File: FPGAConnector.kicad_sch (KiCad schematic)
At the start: 5 parts, among them J4 Conn_02x06_Counter_Clockwise, J5 Conn_02x07_Vertical, J6 To The Zedboard, J8 Conn_02x06_Odd_Even, J9 Conn_02x05_Counter_Clockwise

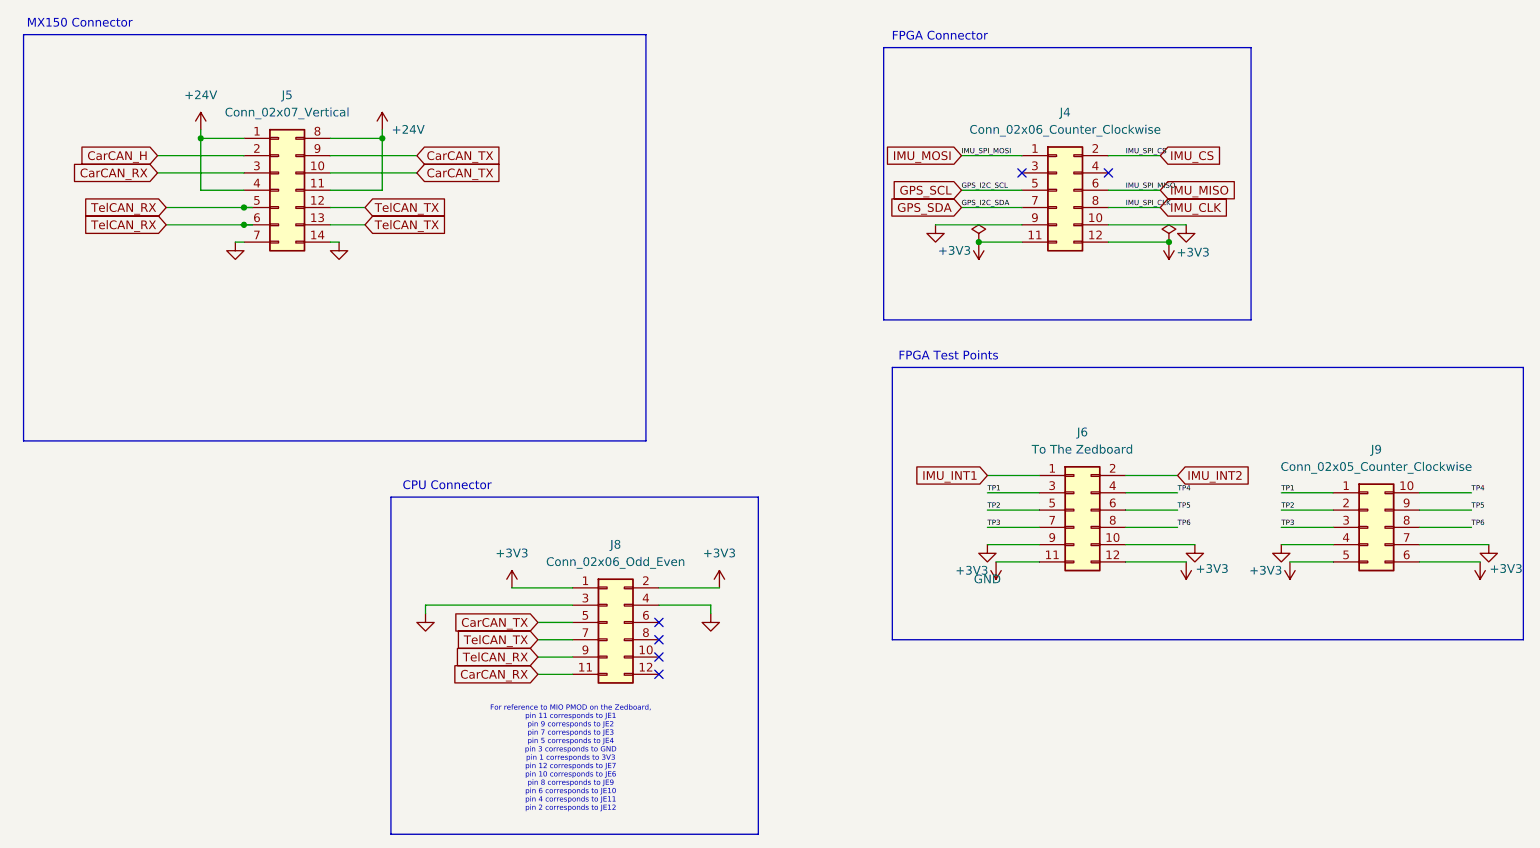
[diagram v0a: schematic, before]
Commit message: more layout
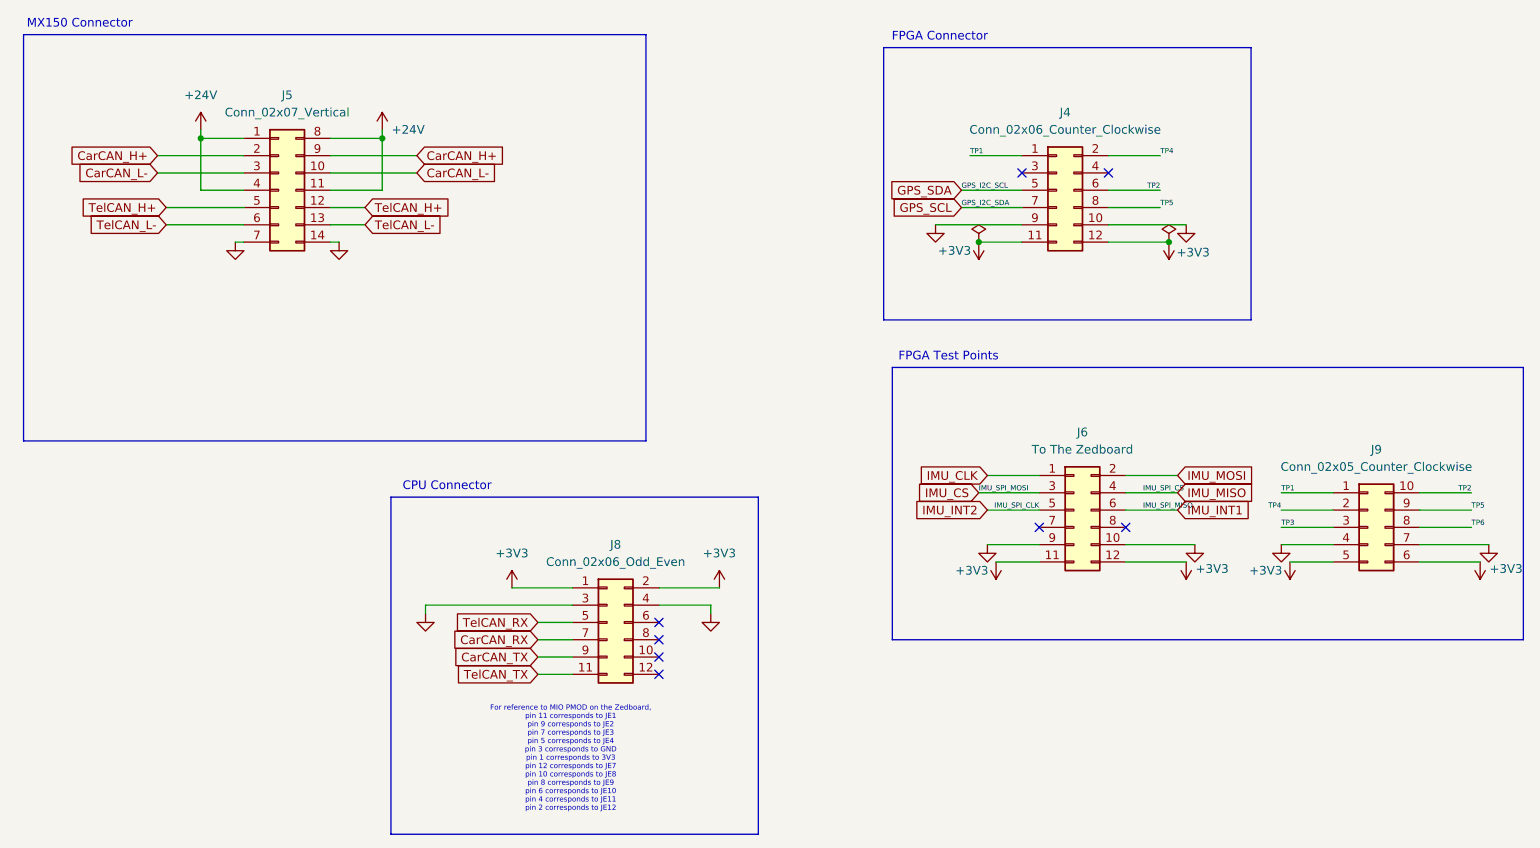
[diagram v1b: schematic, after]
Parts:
- J4: footprint Connector_PinHeader_2.54mm:PinHeader_2x07_P2.54mm_Vertical -> Connector_PinHeader_2.54mm:PinHeader_2x06_P2.54mm_Vertical
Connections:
- net CarCAN_RX: now also J8.7 (Pin_7); no longer J5.3 (Pin_3), J8.11 (Pin_11)
- net CarCAN_TX: now also J8.9 (Pin_9); no longer J5.10 (Pin_10), J5.9 (Pin_9), J8.5 (Pin_5)
- net GPS_SCL: now also J4.7 (Pin_7); no longer J4.5 (Pin_5)
- net GPS_SDA: now also J4.5 (Pin_5); no longer J4.7 (Pin_7)
- net IMU_CLK: now also J6.1 (Pin_1); no longer J4.8 (Pin_8)
- net IMU_CS: now also J6.3 (Pin_2); no longer J4.2 (Pin_2)
- net IMU_INT1: now also J6.6 (Pin_6); no longer J6.1 (Pin_1)
- net IMU_INT2: now also J6.5 (Pin_5); no longer J6.2 (Pin_2)
- net IMU_MISO: now also J6.4 (Pin_4); no longer J4.6 (Pin_6)
- net IMU_MOSI: now also J6.2 (Pin_2); no longer J4.1 (Pin_1)
- net TP1: now also J4.1 (Pin_1); no longer J6.3 (Pin_2)
- net TP2: now also J4.6 (Pin_6), J9.10 (Pin_10); no longer J6.5 (Pin_5), J9.2 (Pin_2)
- net TP3: no longer J6.7 (Pin_7)
- net TP4: now also J4.2 (Pin_2), J9.2 (Pin_2); no longer J6.4 (Pin_4), J9.10 (Pin_10)
- net TP5: now also J4.8 (Pin_8); no longer J6.6 (Pin_6)
- net TP6: no longer J6.8 (Pin_8)
- net TelCAN_RX: now also J8.5 (Pin_5); no longer J5.5 (Pin_5), J5.6 (Pin_6), J8.9 (Pin_9)
- net TelCAN_TX: now also J8.11 (Pin_11); no longer J5.12 (Pin_12), J5.13 (Pin_13), J8.7 (Pin_7)
- net CarCAN_H renamed CarCAN_H+
- net CarCAN_H+: now also J5.9 (Pin_9)
- new net CarCAN_L-: J5.10 (Pin_10), J5.3 (Pin_3)
- new net TelCAN_H+: J5.12 (Pin_12), J5.5 (Pin_5)
- new net TelCAN_L-: J5.13 (Pin_13), J5.6 (Pin_6)
- no-connect marks 6 -> 8
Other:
- note added: "For reference to MIO PMOD on the Zedboard, pin 11 corresponds to JE1 pin 9 corresponds to JE2 pin 7 corresponds to JE3 pin 5 corresponds to JE4 pin 3 corresponds to GND pin 1 corresponds to 3V3 pin 12 corresponds to JE7 pin 10 corresponds to JE8 pin 8 corresponds to JE9 pin 6 corresponds to JE10 pin 4 corresponds to JE11 pin 2 corresponds to JE12"
- note removed: "For reference to MIO PMOD on the Zedboard, pin 11 corresponds to JE1 pin 9 corresponds to JE2 pin 7 corresponds to JE3 pin 5 corresponds to JE4 pin 3 corresponds to GND pin 1 corresponds to 3V3 pin 12 corresponds to JE7 pin 10 corresponds to JE6 pin 8 corresponds to JE9 pin 6 corresponds to JE10 pin 4 corresponds to JE11 pin 2 corresponds to JE12"
